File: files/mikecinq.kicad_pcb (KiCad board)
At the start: 2 copper layers, 226.9 x 108.5 mm, 80 parts, among them SW1 SW_SPST, U1 Nice_Nano_V2

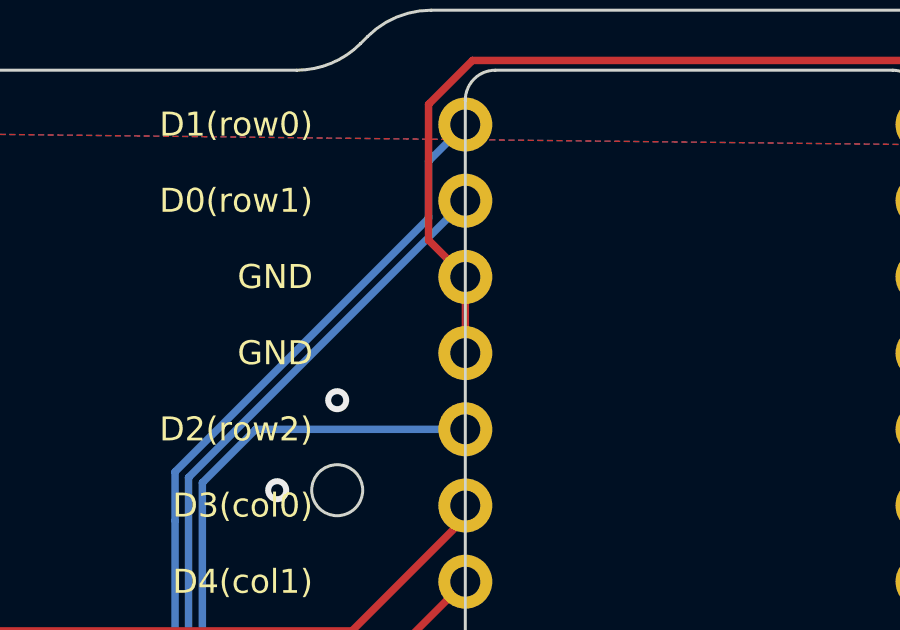
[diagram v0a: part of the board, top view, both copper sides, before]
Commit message: general updates
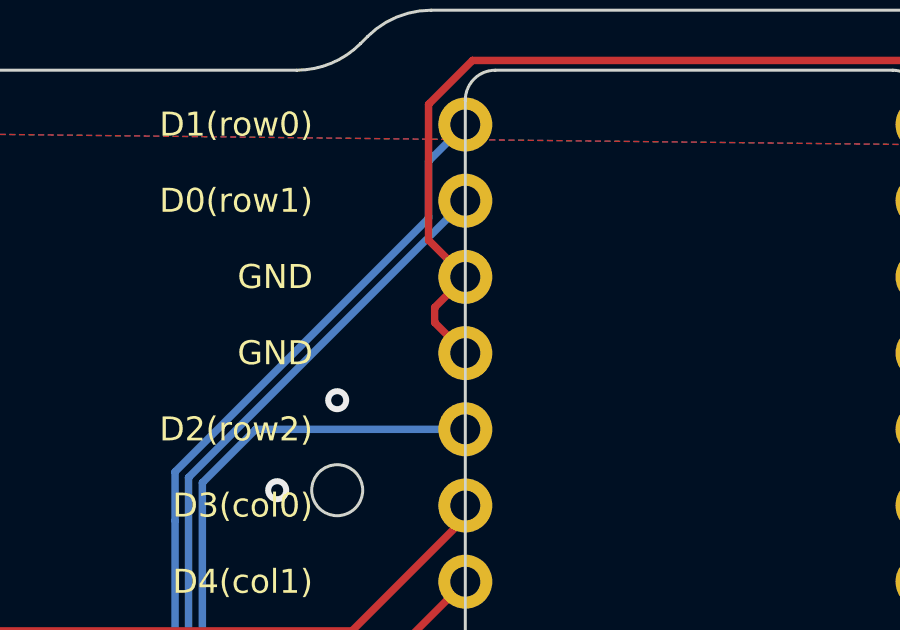
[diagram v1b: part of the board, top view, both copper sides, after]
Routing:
- net GND: track 64.2 -> 65.0 mm
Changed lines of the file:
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@@
 		(tags "resistor")
 		(property "Reference" "R1"
-			(at 2.388268 1.5 360)
+			(at 2.388268 1.5 0)
 			(layer "F.SilkS")
 			(effects
@@
 		)
 		(property "Value" "R"
-			(at 0 0 360)
+			(at 0 0 0)
 			(layer "F.Fab")
 			(effects
@@
 		)
 		(fp_text user "${REFERENCE}"
-			(at 0 0 360)
+			(at 0 0 0)
 			(layer "F.Fab")
 			(effects
@@
 		(tags "inductor")
 		(property "Reference" "FB1"
-			(at 2.799999 0 360)
+			(at 2.799999 0 0)
 			(layer "F.SilkS")
 			(effects
@@
 		)
 		(property "Value" "FerriteBead"
-			(at 0.236032 2.964315 360)
+			(at 0.236032 2.964315 0)
 			(layer "F.Fab")
 			(effects
@@
 		)
 		(fp_text user "${REFERENCE}"
-			(at 0 0 360)
+			(at 0 0 0)
 			(layer "F.Fab")
 			(effects
@@
 		(tags "capacitor")
 		(property "Reference" "C1"
-			(at 2.388266 -1.500001 360)
+			(at 2.388266 -1.500001 0)
 			(layer "F.SilkS")
 			(effects
@@
 		)
 		(property "Value" "C"
-			(at -0.063969 0.064314 360)
+			(at -0.063969 0.064314 0)
 			(layer "F.Fab")
 			(effects
@@
 		)
 		(fp_text user "${REFERENCE}"
-			(at 0 0 360)
+			(at 0 0 0)
 			(layer "F.Fab")
 			(effects
@@
 		)
 		(property "Footprint" "Custom:MSK12C02"
-			(at 0 0 360)
+			(at 0 0 0)
 			(layer "F.Fab")
 			(hide yes)
@@
 		)
 		(property "Datasheet" ""
-			(at 0 0 360)
+			(at 0 0 0)
 			(layer "F.Fab")
 			(hide yes)
@@
 		)
 		(property "Description" "Switch, single pole double throw"
-			(at 0 0 360)
+			(at 0 0 0)
 			(layer "F.Fab")
 			(hide yes)
@@
 	)
 	(segment
+		(start 131.428722 28.660337)
+		(end 130.408722 29.680337)
+		(width 0.25)
+		(layer "F.Cu")
+		(net 54)
+	)
+	(segment
 		(start 153.674405 33.126022)
 		(end 146.668721 26.120338)
@@
 	)
 	(segment
-		(start 131.428722 28.660337)
-		(end 131.428722 31.200337)
+		(start 158.813456 33.138523)
+		(end 158.800955 33.126022)
 		(width 0.25)
 		(layer "F.Cu")
@@
 	)
 	(segment
-		(start 158.813456 33.138523)
-		(end 158.800955 33.126022)
+		(start 130.408722 30.180337)
+		(end 131.428722 31.200337)
 		(width 0.25)
 		(layer "F.Cu")
@@
 		(width 0.25)
 		(layer "F.Cu")
+		(net 54)
+	)
+	(segment
+		(start 130.408722 29.680337)
+		(end 130.408722 30.180337)
+		(width 0.25)
+		(layer "F.Cu")
